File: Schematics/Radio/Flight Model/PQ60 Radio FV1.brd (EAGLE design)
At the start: 42 x 42 mm, 7 parts

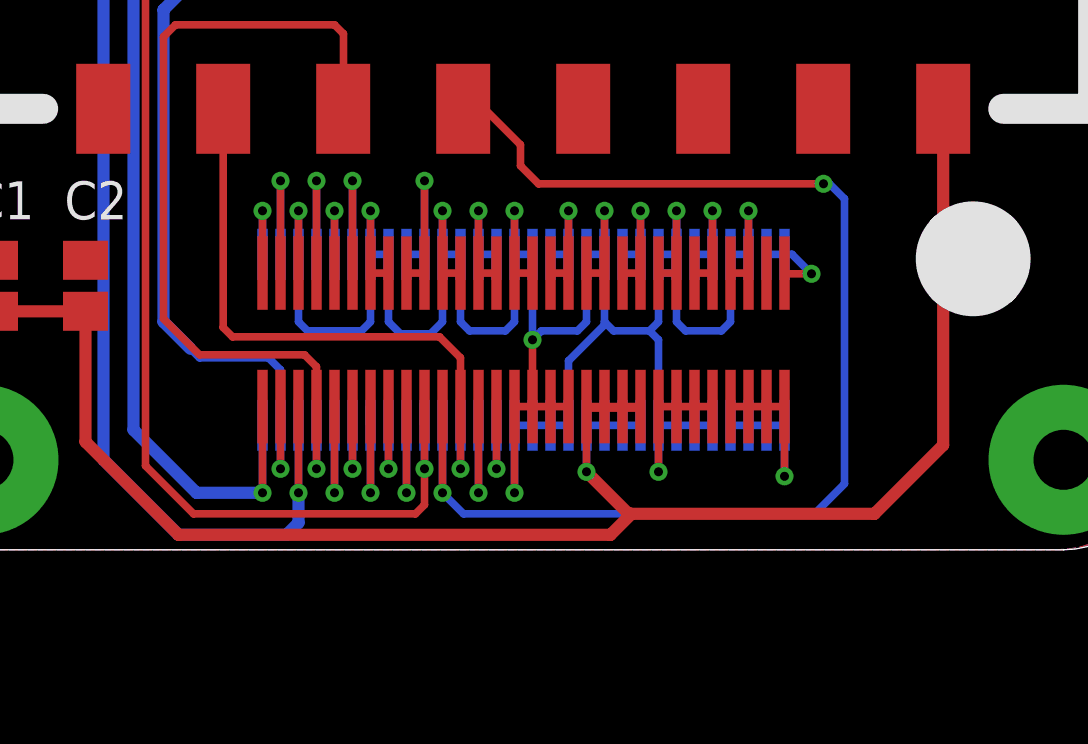
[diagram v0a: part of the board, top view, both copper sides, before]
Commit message: many changes
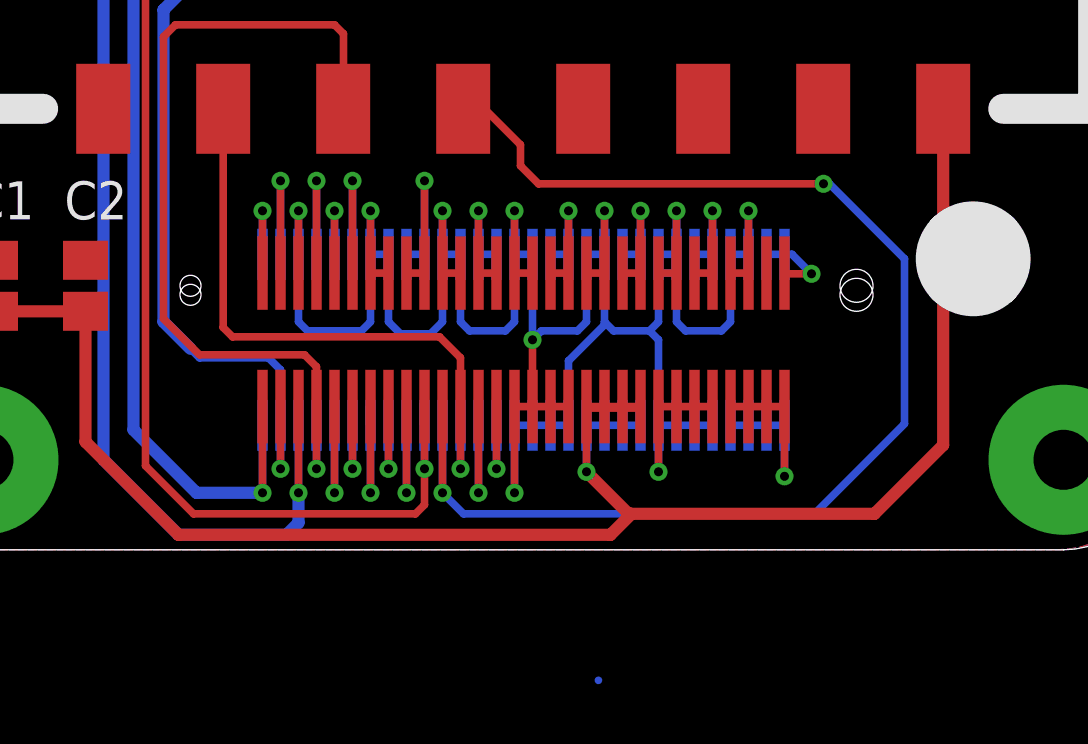
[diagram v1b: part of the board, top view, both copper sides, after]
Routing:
- net GPIO9: track 43.1 -> 44.7 mm
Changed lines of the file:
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@@
 <via x="31" y="12.2" extent="1-16" drill="0.3"/>
 <wire x1="31" y1="12.2" x2="31.2" y2="12.2" width="0.254" layer="16"/>
-<wire x1="31.2" y1="12.2" x2="31.7" y2="11.7" width="0.254" layer="16"/>
-<wire x1="31.7" y1="11.7" x2="31.7" y2="2.2" width="0.254" layer="16"/>
-<wire x1="31.7" y1="2.2" x2="30.7" y2="1.2" width="0.254" layer="16"/>
 <wire x1="30.7" y1="1.2" x2="19" y2="1.2" width="0.254" layer="16"/>
 <wire x1="19" y1="1.2" x2="18.3" y2="1.9" width="0.254" layer="16"/>
+<wire x1="31.2" y1="12.2" x2="33.7" y2="9.7" width="0.254" layer="16"/>
+<wire x1="33.7" y1="9.7" x2="33.7" y2="4.2" width="0.254" layer="16"/>
+<wire x1="33.7" y1="4.2" x2="30.7" y2="1.2" width="0.254" layer="16"/>
 </signal>
 <signal name="GPIO10">
